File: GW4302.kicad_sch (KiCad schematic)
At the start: 80 parts, among them J1 C64, J2 microUSB, J3 JTAG, U1 74AHC245PW, U10 74AHC125PW, U13 CH340G, U2 74AHC245PW, U3 LD1117S33, U4 74AHC245PW, U5 74AHC245PW, U6 74AHC125PW, U8 LCMXO2-640-TG100, U9 W9825G6KH-6, Y1 12M

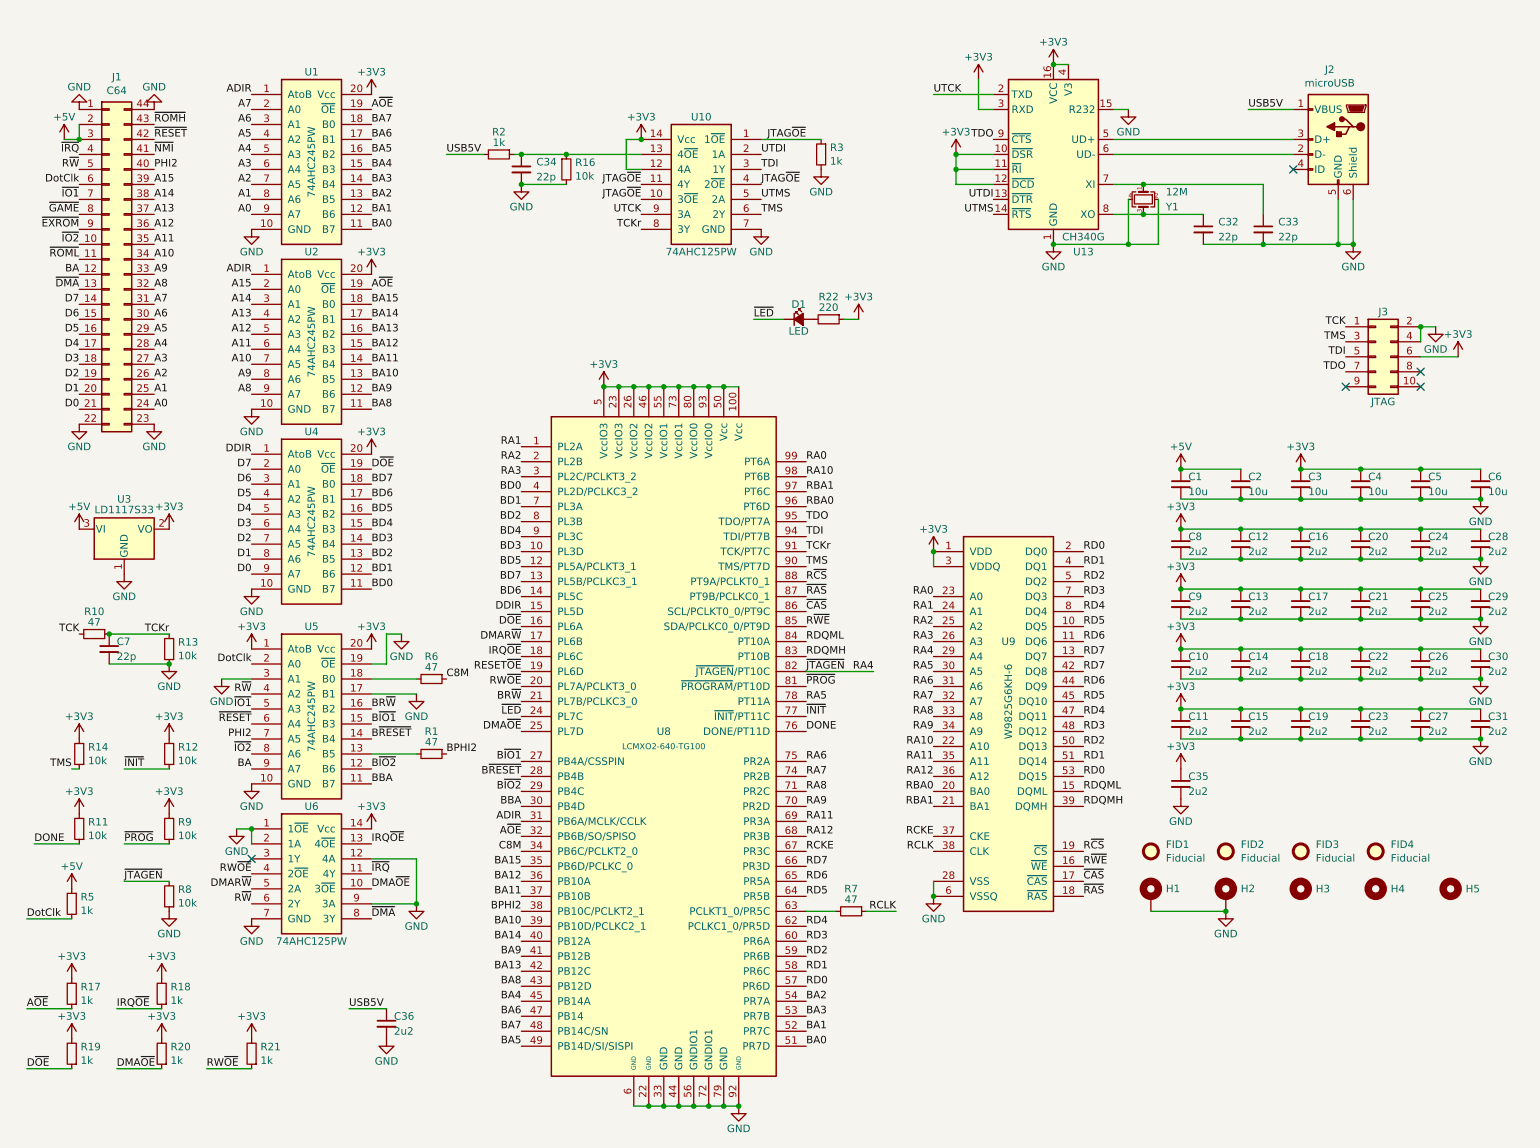
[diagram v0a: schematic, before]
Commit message: New version
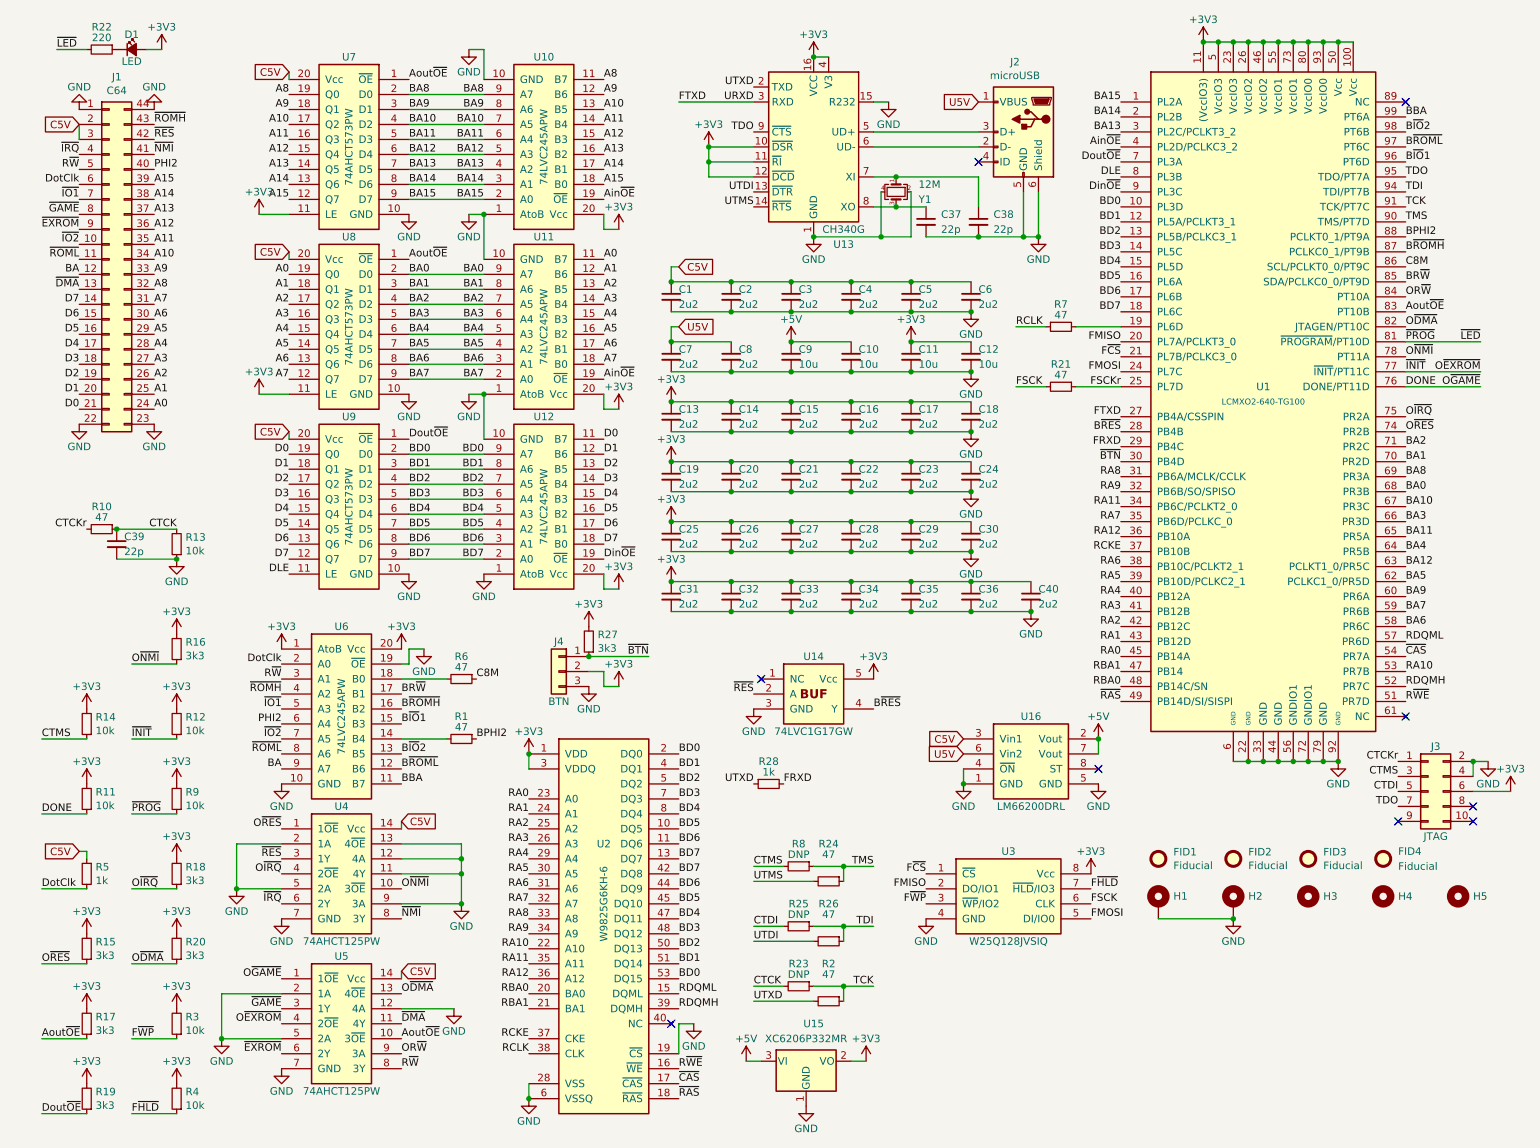
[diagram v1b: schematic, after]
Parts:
- removed U10: 74AHC125PW, stdpads:TSSOP-14_4.4x5mm_P0.65mm, symbol GW_Logic:74125
- removed U3: LD1117S33, stdpads:SOT-223, symbol Regulator_Linear:LD1117S33TR_SOT223
- added C32, C33, C40, C7: 2u2, stdpads:C_0603, symbol Device:C_Small
- added J4: BTN, stdpads:PinHeader_1x03_P2.00mm_Vertical, symbol Connector_Generic:Conn_01x03
- added R15, R27: 3k3, stdpads:R_0603, symbol Device:R_Small
- added R23, R25: DNP, stdpads:R_0603, symbol Device:R_Small
- added R24, R26: 47, stdpads:R_0603, symbol Device:R_Small
- added R28: 1k, stdpads:R_0603, symbol Device:R_Small
- added R4: 10k, stdpads:R_0603, symbol Device:R_Small
- added U14: 74LVC1G17GW, stdpads:SOT-353, symbol GW_Logic:741G07GW
- added U15: XC6206P332MR, stdpads:SOT-23, symbol Regulator_Linear:XC6206PxxxMR
- added U16: LM66200DRL, stdpads:SOT-583, symbol GW_Power:LM66200DCK
- added U3: W25Q128JVSIQ, stdpads:SOIC-8_5.3mm, symbol GW_RAM:SPIFlash-SO-8
- added U5: 74AHCT125PW, stdpads:TSSOP-14_4.4x5mm_P0.65mm, symbol GW_Logic:74125
- added U7, U8, U9: 74AHCT573PW, stdpads:TSSOP-20_4.4x6.5mm_P0.65mm, symbol GW_Logic:74573
- C1, C2, C3, C4, C5, C6: value 10u -> 2u2; footprint stdpads:C_0805 -> stdpads:C_0603; LCSC Part C15850 -> C23630
- C10, C11, C12, C9: value 2u2 -> 10u; footprint stdpads:C_0603 -> stdpads:C_0805; LCSC Part C23630 -> C15850
- C34: value 22p -> 2u2; LCSC Part C1653 -> C23630
- D1: LCSC Part (none) -> C284932
- H1, H2, H3, H4, H5: value (none) -> ~
- J2: LCSC Part C404969 -> C132564
- J3: footprint Connector:Tag-Connect_TC2050-IDC-FP_2x05_P1.27mm_Vertical -> stdpads:Tag-Connect_TC2050-IDC-FP_2x05_P1.27mm_Vertical
- R16: value 10k -> 3k3; LCSC Part C25804 -> C22978
- R17, R18, R19, R20: value 1k -> 3k3; LCSC Part C25804 -> C22978
- R2: value 1k -> 47; LCSC Part C21190 -> C23182
- R21: value 1k -> 47; LCSC Part C25804 -> C23182
- R22: LCSC Part (none) -> C17557
- R3: value 1k -> 10k; LCSC Part C21190 -> C25804
- R8: value 10k -> DNP; LCSC Part C25804 -> (none)
- U1: renamed from U8; LCSC Part (none) -> C1521611
- U10: renamed from U1; value 74AHC245PW -> 74LVC245APW; LCSC Part C132987 -> C7848
- U11: renamed from U2; value 74AHC245PW -> 74LVC245APW; LCSC Part C132987 -> C7848
- U12: renamed from U4; value 74AHC245PW -> 74LVC245APW; LCSC Part C132987 -> C7848
- U4: renamed from U6; value 74AHC125PW -> 74AHCT125PW; LCSC Part C129518 -> C36365
- U6: renamed from U5; value 74AHC245PW -> 74LVC245APW; LCSC Part C132987 -> C7848
- Y1: LCSC Part (none) -> C9002
- renumbered C32 to C37, C33 to C38, C7 to C39, U9 to U2
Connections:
- net RESET~{OE} is gone; now on an unnamed net: U1.19 (PL6D)
- net ~{PROG} is gone; now on net ~{LED}: R9.1, U1.81 (~{PROGRAM}/PT10D)
- net +3V3: now also C34.1, C36.1, D1.2 (A), R16.2, R3.2, U1.11 ((VccIO3)), C32.1, C33.1, C40.1, J4.2 (Pin_2), R15.2, R27.2, R4.2, U14.5 (Vcc), U15.2 (VO), U3.8 (Vcc), U7.11 (LE), U8.11 (LE); no longer C10.1, C3.1, C4.1, C5.1, C6.1, C8.1, C9.1, R21.2, R22.1, U13.3 (RXD), U4.14 (Vcc)
- net +5V: now also C10.1, C9.1, U15.3 (VI), U16.2 (Vout), U16.7 (Vout); no longer C1.1, C2.1, J1.2 (Pin_2), J1.3 (Pin_3), R5.1
- net A0: now also U11.11 (B7), U8.19 (Q0); no longer U10.9 (A7)
- net A1: now also U11.12 (B6), U8.18 (Q1); no longer U10.8 (A6)
- net A10: now also U10.13 (B5), U7.17 (Q2); no longer U11.7 (A5)
- net A11: now also U10.14 (B4), U7.16 (Q3); no longer U11.6 (A4)
- net A12: now also U10.15 (B3), U7.15 (Q4); no longer U11.5 (A3)
- net A13: now also U10.16 (B2), U7.14 (Q5); no longer U11.4 (A2)
- net A14: now also U10.17 (B1), U7.13 (Q6); no longer U11.3 (A1)
- net A15: now also U10.18 (B0), U7.12 (Q7); no longer U11.2 (A0)
- net A2: now also U11.13 (B5), U8.17 (Q2); no longer U10.7 (A5)
- net A3: now also U11.14 (B4), U8.16 (Q3); no longer U10.6 (A4)
- net A4: now also U11.15 (B3), U8.15 (Q4); no longer U10.5 (A3)
- net A5: now also U11.16 (B2), U8.14 (Q5); no longer U10.4 (A2)
- net A6: now also U11.17 (B1), U8.13 (Q6); no longer U10.3 (A1)
- net A7: now also U11.18 (B0), U8.12 (Q7); no longer U10.2 (A0)
- net A8: now also U10.11 (B7), U7.19 (Q0); no longer U11.9 (A7)
- net A9: now also U10.12 (B6), U7.18 (Q1); no longer U11.8 (A6)
- net BA0: now also U1.68 (PR3B), U11.9 (A7), U8.2 (D0); no longer U1.51 (PR7D), U10.11 (B7)
- net BA1: now also U1.70 (PR2D), U11.8 (A6), U8.3 (D1); no longer U1.52 (PR7C), U10.12 (B6)
- net BA10: now also U1.67 (PR3C), U10.7 (A5), U7.4 (D2); no longer U1.39 (PB10D/PCLKC2_1), U11.13 (B5)
- net BA11: now also U1.65 (PR5A), U10.6 (A4), U7.5 (D3); no longer U1.37 (PB10B), U11.14 (B4)
- net BA12: now also U1.63 (PCLKT1_0/PR5C), U10.5 (A3), U7.6 (D4); no longer U1.36 (PB10A), U11.15 (B3)
- net BA13: now also U1.3 (PL2C/PCLKT3_2), U10.4 (A2), U7.7 (D5); no longer U1.42 (PB12C), U11.16 (B2)
- net BA14: now also U1.2 (PL2B), U10.3 (A1), U7.8 (D6); no longer U1.40 (PB12A), U11.17 (B1)
- net BA15: now also U1.1 (PL2A), U10.2 (A0), U7.9 (D7); no longer U1.35 (PB6D/PCLKC_0), U11.18 (B0)
- net BA2: now also U1.71 (PR2C), U11.7 (A5), U8.4 (D2); no longer U1.54 (PR7A), U10.13 (B5)
- net BA3: now also U1.66 (PR3D), U11.6 (A4), U8.5 (D3); no longer U1.53 (PR7B), U10.14 (B4)
- net BA4: now also U1.64 (PR5B), U11.5 (A3), U8.6 (D4); no longer U1.45 (PB14A), U10.15 (B3)
- net BA5: now also U1.62 (PCLKC1_0/PR5D), U11.4 (A2), U8.7 (D5); no longer U1.49 (PB14D/SI/SISPI), U10.16 (B2)
- net BA6: now also U1.58 (PR6C), U11.3 (A1), U8.8 (D6); no longer U1.47 (PB14), U10.17 (B1)
- net BA7: now also U1.59 (PR6B), U11.2 (A0), U8.9 (D7); no longer U1.48 (PB14C/SN), U10.18 (B0)
- net BA8: now also U1.69 (PR3A), U10.9 (A7), U7.2 (D0); no longer U1.43 (PB12D), U11.11 (B7)
- net BA9: now also U1.60 (PR6A), U10.8 (A6), U7.3 (D1); no longer U1.41 (PB12B), U11.12 (B6)
- net BBA: now also U1.99 (PT6A); no longer U1.30 (PB4D)
- net BD0: now also U1.10 (PL3D), U12.9 (A7), U2.2 (DQ0), U2.53 (DQ15), U9.2 (D0); no longer U1.4 (PL2D/PCLKC3_2), U12.11 (B7)
- net BD1: now also U1.12 (PL5A/PCLKT3_1), U12.8 (A6), U2.4 (DQ1), U2.51 (DQ14), U9.3 (D1); no longer U1.7 (PL3A), U12.12 (B6)
- net BD2: now also U1.13 (PL5B/PCLKC3_1), U12.7 (A5), U2.5 (DQ2), U2.50 (DQ13), U9.4 (D2); no longer U1.8 (PL3B), U12.13 (B5)
- net BD3: now also U1.14 (PL5C), U12.6 (A4), U2.48 (DQ12), U2.7 (DQ3), U9.5 (D3); no longer U1.10 (PL3D), U12.14 (B4)
- net BD4: now also U1.15 (PL5D), U12.5 (A3), U2.47 (DQ11), U2.8 (DQ4), U9.6 (D4); no longer U1.9 (PL3C), U12.15 (B3)
- net BD5: now also U1.16 (PL6A), U12.4 (A2), U2.10 (DQ5), U2.45 (DQ10), U9.7 (D5); no longer U1.12 (PL5A/PCLKT3_1), U12.16 (B2)
- net BD6: now also U1.17 (PL6B), U12.3 (A1), U2.11 (DQ6), U2.44 (DQ9), U9.8 (D6); no longer U1.14 (PL5C), U12.17 (B1)
- net BD7: now also U1.18 (PL6C), U12.2 (A0), U2.13 (DQ7), U2.42 (DQ8), U9.9 (D7); no longer U1.13 (PL5B/PCLKC3_1), U12.18 (B0)
- net BPHI2: now also U1.88 (PCLKT0_1/PT9A); no longer U1.38 (PB10C/PCLKT2_1)
- net BR~{W}: now also U1.85 (SDA/PCLKC0_0/PT9D), U6.17 (B1); no longer U1.21 (PL7B/PCLKC3_0), U6.16 (B2)
- net C8M: now also U1.86 (SCL/PCLKT0_0/PT9C); no longer U1.34 (PB6C/PCLKT2_0)
- net D0: now also U12.11 (B7), U9.19 (Q0); no longer U12.9 (A7)
- net D1: now also U12.12 (B6), U9.18 (Q1); no longer U12.8 (A6)
- net D2: now also U12.13 (B5), U9.17 (Q2); no longer U12.7 (A5)
- net D3: now also U12.14 (B4), U9.16 (Q3); no longer U12.6 (A4)
- net D4: now also U12.15 (B3), U9.15 (Q4); no longer U12.5 (A3)
- net D5: now also U12.16 (B2), U9.14 (Q5); no longer U12.4 (A2)
- net D6: now also U12.17 (B1), U9.13 (Q6); no longer U12.3 (A1)
- net D7: now also U12.18 (B0), U9.12 (Q7); no longer U12.2 (A0)
- net DONE: now also U5.1 (1~{OE})
- net GND: now also U10.1 (AtoB), U11.1 (AtoB), U12.1 (AtoB), U2.19 (~{CS}), U4.11 (4Y), U4.13 (4~{OE}), U4.5 (2A), C32.2, C33.2, C40.2, C7.2, J4.3 (Pin_3), U14.3 (GND), U15.1 (GND), U16.1 (GND), U16.4 (~{ON}), U16.5 (GND), U3.4 (GND), U5.12 (4A), U5.2 (1A), U5.5 (2A), U5.7 (GND), U7.10 (GND), U8.10 (GND), U9.10 (GND); no longer R16.2, R3.2, R8.1, U4.1 (1~{OE}), U6.17 (B1), U6.3 (A1)
- net PHI2: now also U6.6 (A4); no longer U6.7 (A5)
- net RA0: now also U1.45 (PB14A); no longer U1.99 (PT6A)
- net RA1: now also U1.43 (PB12D); no longer U1.1 (PL2A)
- net RA10: now also U1.53 (PR7B); no longer U1.98 (PT6B)
- net RA11: now also U1.34 (PB6C/PCLKT2_0); no longer U1.69 (PR3A)
- net RA12: now also U1.36 (PB10A); no longer U1.68 (PR3B)
- net RA2: now also U1.42 (PB12C); no longer U1.2 (PL2B)
- net RA3: now also U1.41 (PB12B); no longer U1.3 (PL2C/PCLKT3_2)
- net RA4: now also U1.40 (PB12A); no longer R8.2, U1.82 (~{JTAGEN}/PT10C)
- net RA5: now also U1.39 (PB10D/PCLKC2_1); no longer U1.78 (PT11A)
- net RA6: now also U1.38 (PB10C/PCLKT2_1); no longer U1.75 (PR2A)
- net RA7: now also U1.35 (PB6D/PCLKC_0); no longer U1.74 (PR2B)
- net RA8: now also U1.31 (PB6A/MCLK/CCLK); no longer U1.71 (PR2C)
- net RA9: now also U1.32 (PB6B/SO/SPISO); no longer U1.70 (PR2D)
- net RBA0: now also U1.48 (PB14C/SN); no longer U1.96 (PT6D)
- net RBA1: now also U1.47 (PB14); no longer U1.97 (PT6C)
- net RCKE: now also U1.37 (PB10B); no longer U1.67 (PR3C)
- net RDQMH: now also U1.52 (PR7C); no longer U1.83 (PT10B)
- net RDQML: now also U1.57 (PR6D); no longer U1.84 (PT10A)
- net R~{WE}: now also U1.51 (PR7D); no longer U1.85 (SDA/PCLKC0_0/PT9D)
- net R~{W}: now also U6.3 (A1), U5.8 (3Y); no longer U4.6 (2Y), U6.4 (A2)
- net TCK: now also R2.1, U1.91 (TCK/PT7C), R23.1; no longer J3.1 (Pin_1), R10.2
- net TDI: now also R25.1, R26.1; no longer J3.5 (Pin_5)
- net TMS: now also R8.1, R24.1; no longer J3.3 (Pin_3), R14.1
- net UTDI: now also R26.2
- net UTMS: now also R24.2
- net ~{CAS}: now also U1.54 (PR7A); no longer U1.86 (SCL/PCLKT0_0/PT9C)
- net ~{DMA}: now also U5.11 (4Y); no longer U4.8 (3Y)
- net ~{EXROM}: now also U5.6 (2Y)
- net ~{GAME}: now also U5.3 (1Y)
- net ~{IO2}: now also U6.7 (A5); no longer U6.8 (A6)
- net ~{IRQ}: now also U4.6 (2Y); no longer U4.11 (4Y)
- net ~{LED}: now also R22.2; no longer D1.1 (K), U1.24 (PL7C)
- net ~{NMI}: now also U4.8 (3Y)
- net ~{RAS}: now also U1.49 (PB14D/SI/SISPI); no longer U1.87 (PT9B/PCLKC0_1)
- net ~{ROMH}: now also U6.4 (A2)
- net ~{ROML}: now also U6.8 (A6)
- net at R1.2: now also U6.14 (B4); no longer U6.13 (B5)
- net ~{RES}: now reaches U4.3 (1Y)
- net ~{RES}: now also J1.42 (Pin_42), U14.2 (A)
- net at R7.2: no longer U1.63 (PCLKT1_0/PR5C)
- removed net ADIR: U1.31 (PB6A/MCLK/CCLK), U10.1 (AtoB), U11.1 (AtoB)
- net A~{OE} renamed Ain~{OE}
- net Ain~{OE}: now also U1.4 (PL2D/PCLKC3_2); no longer R17.1, U1.32 (PB6B/SO/SPISO)
- net B~{IO1} renamed B~{IO}1
- net B~{IO}1: now also U1.96 (PT6D); no longer U1.27 (PB4A/CSSPIN)
- net B~{IO2} renamed B~{ROML}
- net B~{ROML}: now also U1.97 (PT6C); no longer U1.29 (PB4C)
- net B~{RESET} renamed B~{RES}
- net B~{RES}: now also U14.4 (Y); no longer U6.14 (B4)
- removed net DDIR: U1.15 (PL5D), U12.1 (AtoB)
- removed net DMAR~{W}: U1.17 (PL6B), U4.5 (2A)
- removed net DMA~{OE}: R20.1, U1.25 (PL7D), U4.10 (3~{OE})
- removed net D~{OE}: R19.1, U1.16 (PL6A), U12.19 (~{OE})
- removed net IRQ~{OE}: R18.1, U1.18 (PL6C), U4.13 (4~{OE})
- net JTAG~{OE} renamed F~{WP}
- net F~{WP}: now also U3.3 (~{WP}/IO2)
- removed net RD0: U1.57 (PR6D), U2.2 (DQ0), U2.53 (DQ15)
- removed net RD1: U1.58 (PR6C), U2.4 (DQ1), U2.51 (DQ14)
- removed net RD2: U1.59 (PR6B), U2.5 (DQ2), U2.50 (DQ13)
- removed net RD3: U1.60 (PR6A), U2.48 (DQ12), U2.7 (DQ3)
- removed net RD4: U1.62 (PCLKC1_0/PR5D), U2.47 (DQ11), U2.8 (DQ4)
- removed net RD5: U1.64 (PR5B), U2.10 (DQ5), U2.45 (DQ10)
- removed net RD6: U1.65 (PR5A), U2.11 (DQ6), U2.44 (DQ9)
- removed net RD7: U1.66 (PR3D), U2.13 (DQ7), U2.42 (DQ8)
- removed net RW~{OE}: R21.1, U1.20 (PL7A/PCLKT3_0), U4.4 (2~{OE})
- removed net R~{CS}: U1.88 (PT9A/PCLKT0_1), U2.19 (~{CS})
- net TCKr renamed CTCK
- net CTCK: now also R23.2; no longer U1.91 (TCK/PT7C)
- removed net USB5V: C36.1, J2.1 (VBUS), R2.2
- net UTCK renamed UTXD
- net UTXD: now also R2.2, R28.1
- net ~{INIT} renamed O~{EXROM}
- net O~{EXROM}: now also U5.4 (2~{OE})
- removed net ~{RESET}: J1.42 (Pin_42), U6.6 (A4)
- new net: D1.1 (K), R22.1
- new net Aout~{OE}: R17.1, U1.83 (PT10B), U5.10 (3~{OE}), U7.1 (~{OE}), U8.1 (~{OE})
- new net B~{IO}2: U1.98 (PT6B), U6.13 (B5)
- new net B~{ROMH}: U1.87 (PCLKC0_1/PT9B), U6.16 (B2)
- new net C5V: C1.1, C2.1, C3.1, C4.1, C5.1, C6.1, J1.2 (Pin_2), J1.3 (Pin_3), R5.1, U16.3 (Vin1), U4.14 (Vcc), U5.14 (Vcc), U7.20 (Vcc), U8.20 (Vcc), U9.20 (Vcc)
- new net CTCKr: J3.1 (Pin_1), R10.2
- new net CTDI: J3.5 (Pin_5), R25.2
- new net CTMS: J3.3 (Pin_3), R14.1, R8.2
- new net DLE: U1.8 (PL3B), U9.11 (LE)
- new net Din~{OE}: U1.9 (PL3C), U12.19 (~{OE})
- new net Dout~{OE}: R19.1, U1.7 (PL3A), U9.1 (~{OE})
- new net FMISO: U1.20 (PL7A/PCLKT3_0), U3.2 (DO/IO1)
- new net FMOSI: U1.24 (PL7C), U3.5 (DI/IO0)
- new net FRXD: R28.2, U1.29 (PB4C)
- new net FSCK: R21.2, U3.6 (CLK)
- new net FSCKr: R21.1, U1.25 (PL7D)
- new net FTXD: U1.27 (PB4A/CSSPIN), U13.3 (RXD)
- new net F~{CS}: U1.21 (PL7B/PCLKC3_0), U3.1 (~{CS})
- new net F~{HLD}: R4.1, U3.7 (~{HLD}/IO3)
- new net OR~{W}: U1.84 (PT10A), U5.9 (3A)
- new net O~{DMA}: R20.1, U1.82 (JTAGEN/PT10C), U5.13 (4~{OE})
- new net O~{IRQ}: R18.1, U1.75 (PR2A), U4.4 (2~{OE})
- new net O~{NMI}: R16.1, U1.78 (PT11A), U4.10 (3~{OE})
- new net O~{RES}: R15.1, U1.74 (PR2B), U4.1 (1~{OE})
- new net U5V: C7.1, C8.1, J2.1 (VBUS), U16.6 (Vin2)
- new net ~{BTN}: J4.1 (Pin_1), R27.1, U1.30 (PB4D)
- no-connect marks 5 -> 9
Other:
- moved on the sheet: C37, C38, C39, D1, FID1, FID2, FID3, FID4, H1, H2, H3, H4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
